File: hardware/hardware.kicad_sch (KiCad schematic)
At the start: 89 parts, among them U1 NE555P, U2 LM386, U3 LM3914V

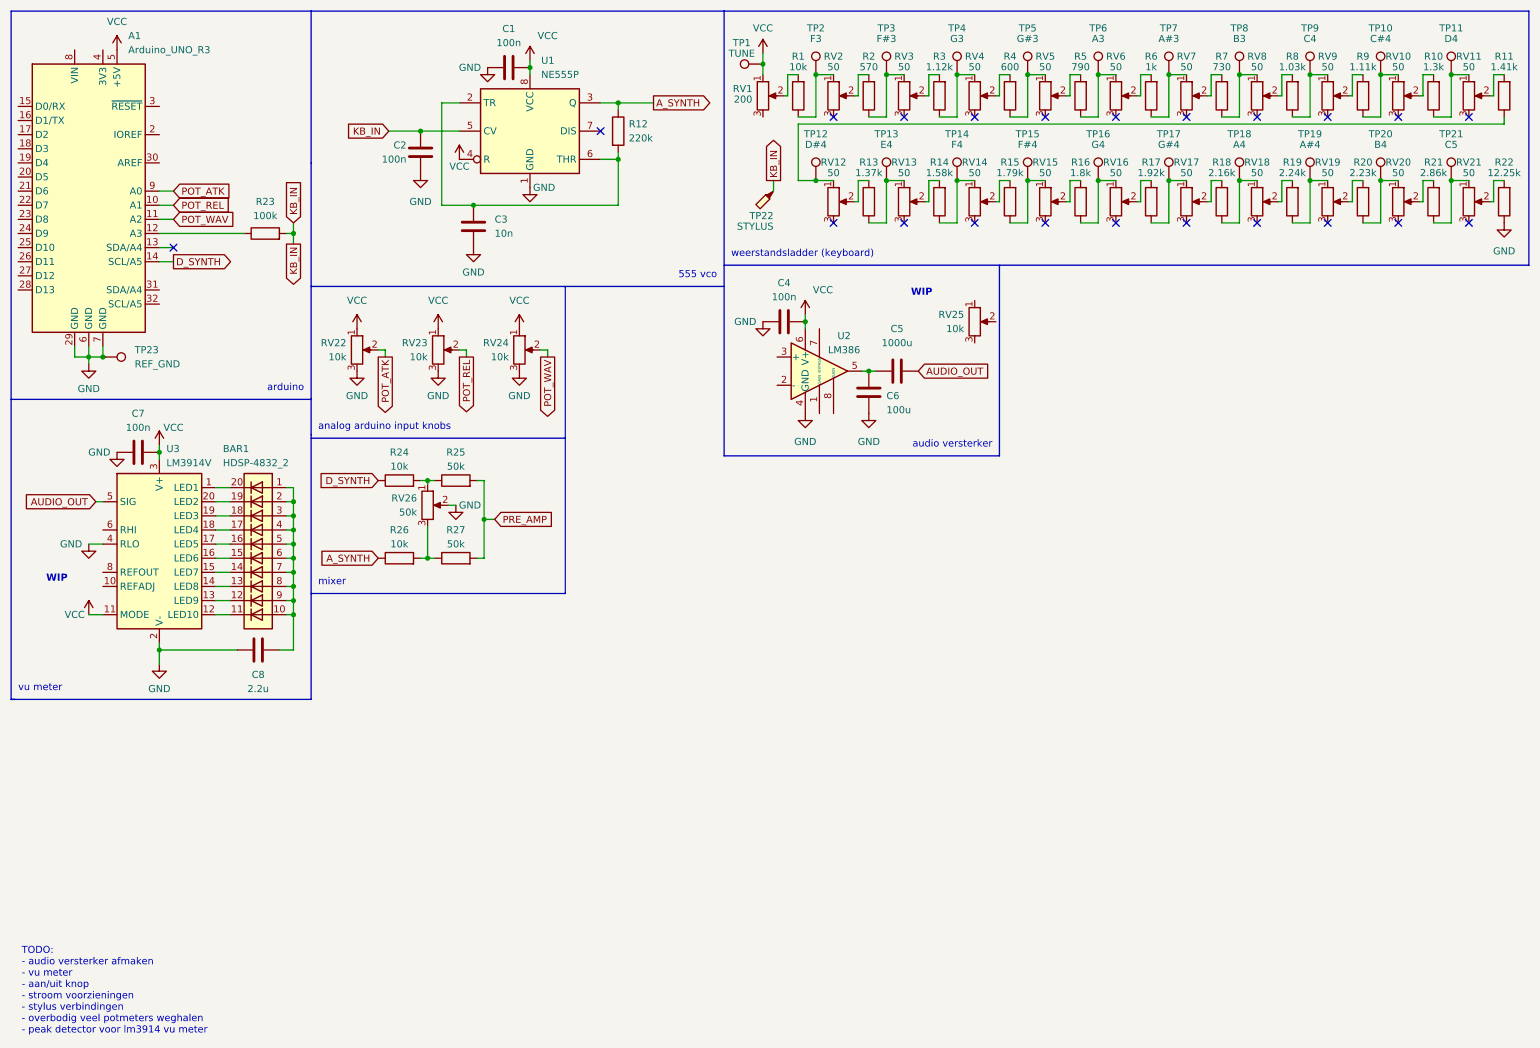
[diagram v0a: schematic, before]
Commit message: more schematics
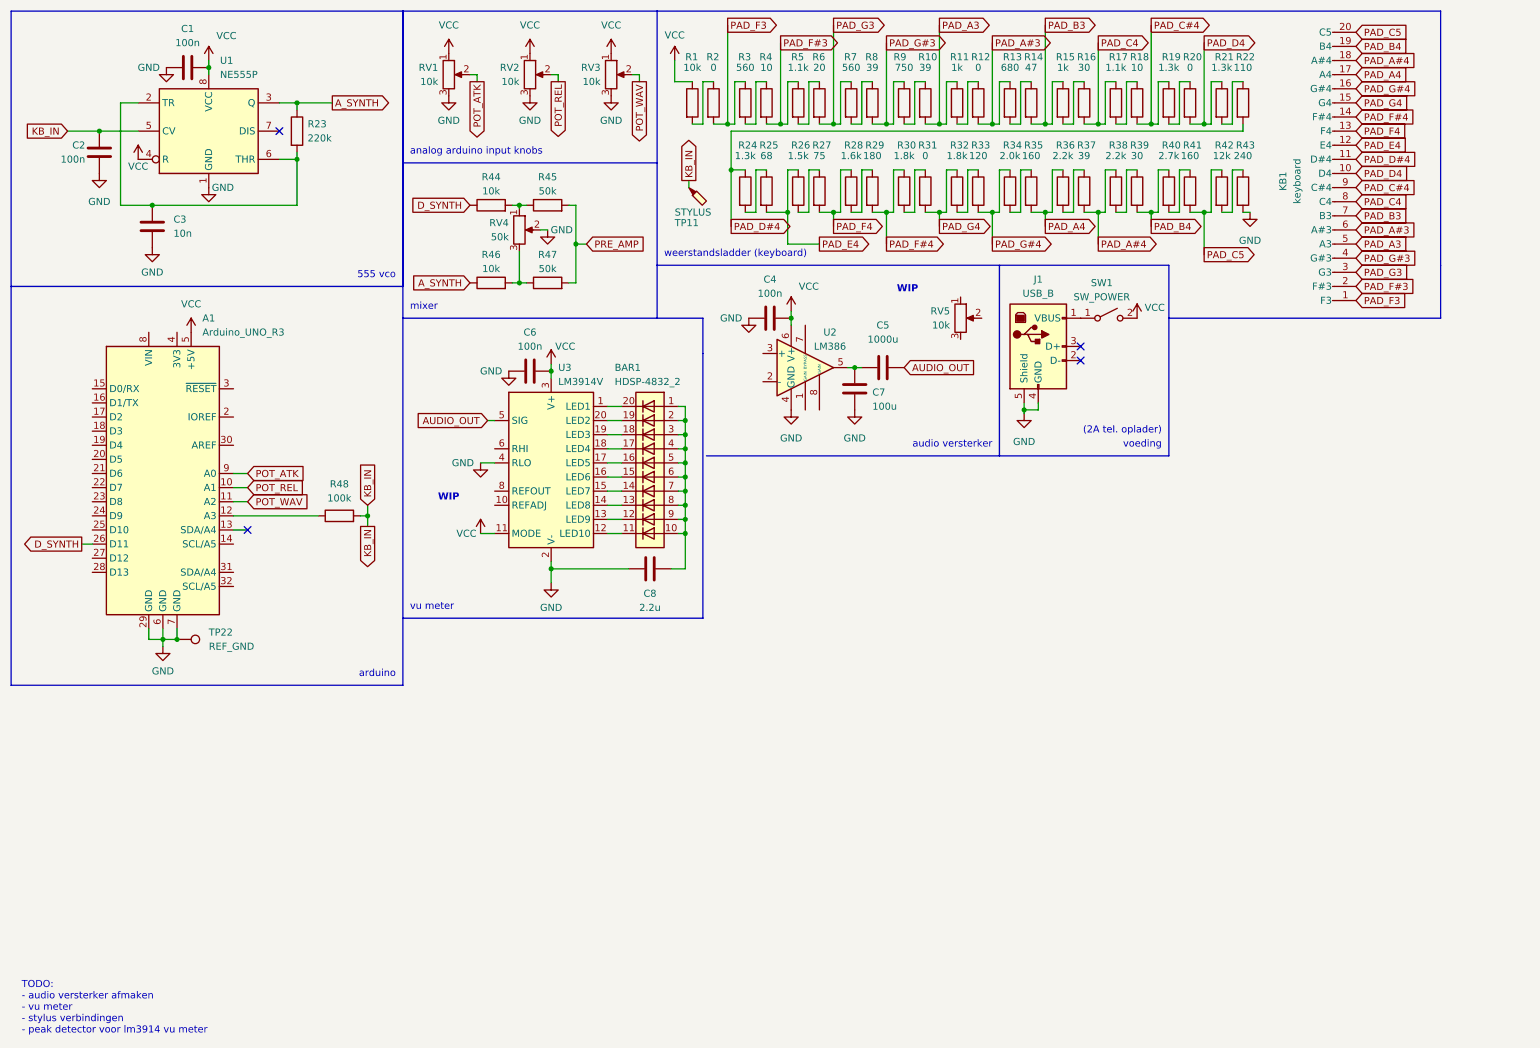
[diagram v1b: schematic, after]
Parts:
- removed RV1: 200, Potentiometer_THT:Potentiometer_ACP_CA9-V10_Vertical, symbol Device:R_Potentiometer
- removed RV10, RV11, RV12, RV13, RV14, RV15, RV16, RV17, RV18, RV19, RV2, RV20, RV21, RV3, RV4, RV5, RV6, RV7, RV8, RV9: 50, Potentiometer_THT:Potentiometer_ACP_CA9-V10_Vertical, symbol Device:R_Potentiometer
- removed TP1: TUNE, symbol Connector:TestPoint
- removed TP10: C#4, symbol Connector:TestPoint
- removed TP11: D4, symbol Connector:TestPoint
- removed TP12: D#4, symbol Connector:TestPoint
- removed TP13: E4, symbol Connector:TestPoint
- removed TP14: F4, symbol Connector:TestPoint
- removed TP15: F#4, symbol Connector:TestPoint
- removed TP16: G4, symbol Connector:TestPoint
- removed TP17: G#4, symbol Connector:TestPoint
- removed TP18: A4, symbol Connector:TestPoint
- removed TP19: A#4, symbol Connector:TestPoint
- removed TP2: F3, symbol Connector:TestPoint
- removed TP20: B4, symbol Connector:TestPoint
- removed TP21: C5, symbol Connector:TestPoint
- removed TP3: F#3, symbol Connector:TestPoint
- removed TP4: G3, symbol Connector:TestPoint
- removed TP5: G#3, symbol Connector:TestPoint
- removed TP6: A3, symbol Connector:TestPoint
- removed TP7: A#3, symbol Connector:TestPoint
- removed TP8: B3, symbol Connector:TestPoint
- removed TP9: C4, symbol Connector:TestPoint
- added J1: USB_B, symbol Connector:USB_B
- added KB1: keyboard, keyboard:keyboard, symbol keyboard:keyboard
- added R12, R31: 0, Resistor_THT:R_Axial_DIN0207_L6.3mm_D2.5mm_P10.16mm_Horizontal, symbol Device:R
- added R24: 1.3k, Resistor_THT:R_Axial_DIN0207_L6.3mm_D2.5mm_P10.16mm_Horizontal, symbol Device:R
- added R25: 68, Resistor_THT:R_Axial_DIN0207_L6.3mm_D2.5mm_P10.16mm_Horizontal, symbol Device:R
- added R26: 1.5k, Resistor_THT:R_Axial_DIN0207_L6.3mm_D2.5mm_P10.16mm_Horizontal, symbol Device:R
- added R27: 75, Resistor_THT:R_Axial_DIN0207_L6.3mm_D2.5mm_P10.16mm_Horizontal, symbol Device:R
- added R28: 1.6k, Resistor_THT:R_Axial_DIN0207_L6.3mm_D2.5mm_P10.16mm_Horizontal, symbol Device:R
- added R29: 180, Resistor_THT:R_Axial_DIN0207_L6.3mm_D2.5mm_P10.16mm_Horizontal, symbol Device:R
- added R30, R32: 1.8k, Resistor_THT:R_Axial_DIN0207_L6.3mm_D2.5mm_P10.16mm_Horizontal, symbol Device:R
- added R33: 120, Resistor_THT:R_Axial_DIN0207_L6.3mm_D2.5mm_P10.16mm_Horizontal, symbol Device:R
- added R34: 2.0k, Resistor_THT:R_Axial_DIN0207_L6.3mm_D2.5mm_P10.16mm_Horizontal, symbol Device:R
- added R35, R41: 160, Resistor_THT:R_Axial_DIN0207_L6.3mm_D2.5mm_P10.16mm_Horizontal, symbol Device:R
- added R36, R38: 2.2k, Resistor_THT:R_Axial_DIN0207_L6.3mm_D2.5mm_P10.16mm_Horizontal, symbol Device:R
- added R37: 39, Resistor_THT:R_Axial_DIN0207_L6.3mm_D2.5mm_P10.16mm_Horizontal, symbol Device:R
- added R39: 30, Resistor_THT:R_Axial_DIN0207_L6.3mm_D2.5mm_P10.16mm_Horizontal, symbol Device:R
- added R40: 2.7k, Resistor_THT:R_Axial_DIN0207_L6.3mm_D2.5mm_P10.16mm_Horizontal, symbol Device:R
- added R42: 12k, Resistor_THT:R_Axial_DIN0207_L6.3mm_D2.5mm_P10.16mm_Horizontal, symbol Device:R
- added R43: 240, Resistor_THT:R_Axial_DIN0207_L6.3mm_D2.5mm_P10.16mm_Horizontal, symbol Device:R
- added SW1: SW_POWER, symbol Switch:SW_SPST
- R10: value 1.3k -> 39
- R11: value 1.41k -> 1k
- R13: value 1.37k -> 680
- R14: value 1.58k -> 47
- R15: value 1.79k -> 1k
- R16: value 1.8k -> 30
- R17: value 1.92k -> 1.1k
- R18: value 2.16k -> 10
- R19: value 2.24k -> 1.3k
- R2: value 570 -> 0
- R20: value 2.23k -> 0
- R21: value 2.86k -> 1.3k
- R22: value 12.25k -> 110
- R3: value 1.12k -> 560
- R4: value 600 -> 10
- R5: value 790 -> 1.1k
- R6: value 1k -> 20
- R7: value 730 -> 560
- R8: value 1.03k -> 39
- R9: value 1.11k -> 750
- renumbered C7 to C6, C6 to C7, R12 to R23, R24 to R44, R25 to R45, R26 to R46, R27 to R47, R23 to R48, RV22 to RV1, RV23 to RV2, RV24 to RV3, RV26 to RV4, RV25 to RV5, TP22 to TP11, TP23 to TP22
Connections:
- net D_SYNTH: now also A1.26 (D11); no longer A1.14 (SCL/A5)
- net GND: now also J1.4 (GND), J1.5 (Shield), R43.2; no longer R22.1
- net VCC: now also R1.1, SW1.2 (B)
- net at R18.1: now also R17.2
- net at R19.2: now also R20.1
- net PAD_C#4: now reaches R19.1
- net PAD_C#4: now also R18.2, KB1.9 (C#4)
- net PAD_A3: now reaches R11.1
- net PAD_A3: now also R10.2, KB1.5 (A3)
- net at R11.2: now also R12.1
- net at R14.1: now also R13.2
- net at R15.2: now also R16.1
- net at R6.1: now also R5.2
- net PAD_B3: now reaches R15.1
- net PAD_B3: now also R14.2, KB1.7 (B3)
- net PAD_C4: now reaches R17.1
- net PAD_C4: now also R16.2, KB1.8 (C4)
- net PAD_G3: now reaches R7.1
- net PAD_G3: now also R6.2, KB1.3 (G3)
- net PAD_A#3: now reaches R13.1
- net PAD_A#3: now also KB1.6 (A#3), R12.2
- net PAD_F#3: now reaches R5.1
- net PAD_F#3: now also R4.2, KB1.2 (F#3)
- net at R21.2: now also R22.1
- net PAD_D4: now reaches R20.2
- net PAD_D4: now also R21.1, KB1.10 (D4)
- net at R4.1: now also R3.2
- net at R8.1: now also R7.2
- net PAD_G#3: now reaches R8.2
- net PAD_G#3: now also R9.1, KB1.4 (G#3)
- net at R10.1: now also R9.2
- net PAD_F3: now reaches R3.1
- net PAD_F3: now also R2.2, KB1.1 (F3)
- net at R1.2: now also R2.1
- net PAD_D#4: now reaches R22.2
- net PAD_D#4: now also KB1.11 (D#4), R24.1
- new net: R24.2, R25.1
- new net: R26.2, R27.1
- new net: R28.2, R29.1
- new net: R42.2, R43.1
- new net: R32.2, R33.1
- new net: R36.2, R37.1
- new net: R34.2, R35.1
- new net: J1.1 (VBUS), SW1.1 (A)
- new net: R30.2, R31.1
- new net: R38.2, R39.1
- new net: R40.2, R41.1
- new net PAD_A#4: KB1.18 (A#4), R37.2, R38.1
- new net PAD_A4: KB1.17 (A4), R35.2, R36.1
- new net PAD_B4: KB1.19 (B4), R39.2, R40.1
- new net PAD_C5: KB1.20 (C5), R41.2, R42.1
- new net PAD_E4: KB1.12 (E4), R25.2, R26.1
- new net PAD_F#4: KB1.14 (F#4), R29.2, R30.1
- new net PAD_F4: KB1.13 (F4), R27.2, R28.1
- new net PAD_G#4: KB1.16 (G#4), R33.2, R34.1
- new net PAD_G4: KB1.15 (G4), R31.2, R32.1
- no-connect marks 22 -> 4
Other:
- note added: "(2A tel. oplader)"
- note added: "TODO: - audio versterker afmaken - vu meter - stylus verbindingen - peak detector voor lm3914 vu meter"
- note added: "voeding"
- note removed: "TODO: - audio versterker afmaken - vu meter - aan/uit knop - stroom voorzieningen - stylus verbindingen - overbodig veel potmeters weghalen - peak detector voor lm3914 vu meter"
- moved on the sheet: A1, BAR1, C1, C2, C3, C4, C5, C6, C7, C8, R23, R44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
